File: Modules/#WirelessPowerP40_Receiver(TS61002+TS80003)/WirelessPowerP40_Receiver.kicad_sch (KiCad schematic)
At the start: 123 parts, among them J2 I2C, J3 I2C, J4 Coil Therm, J5 COIL 20uH, J6 Conn_01x02_Male, J7 Conn_01x02_Male, U1 TS30041, U2 TS94033, U3 74LVC1G66, U4 TS61002, U5 TS80003, U6 BSC0993ND, U7 BSC0993ND, U8 max31740, U9 CSD16406Q3

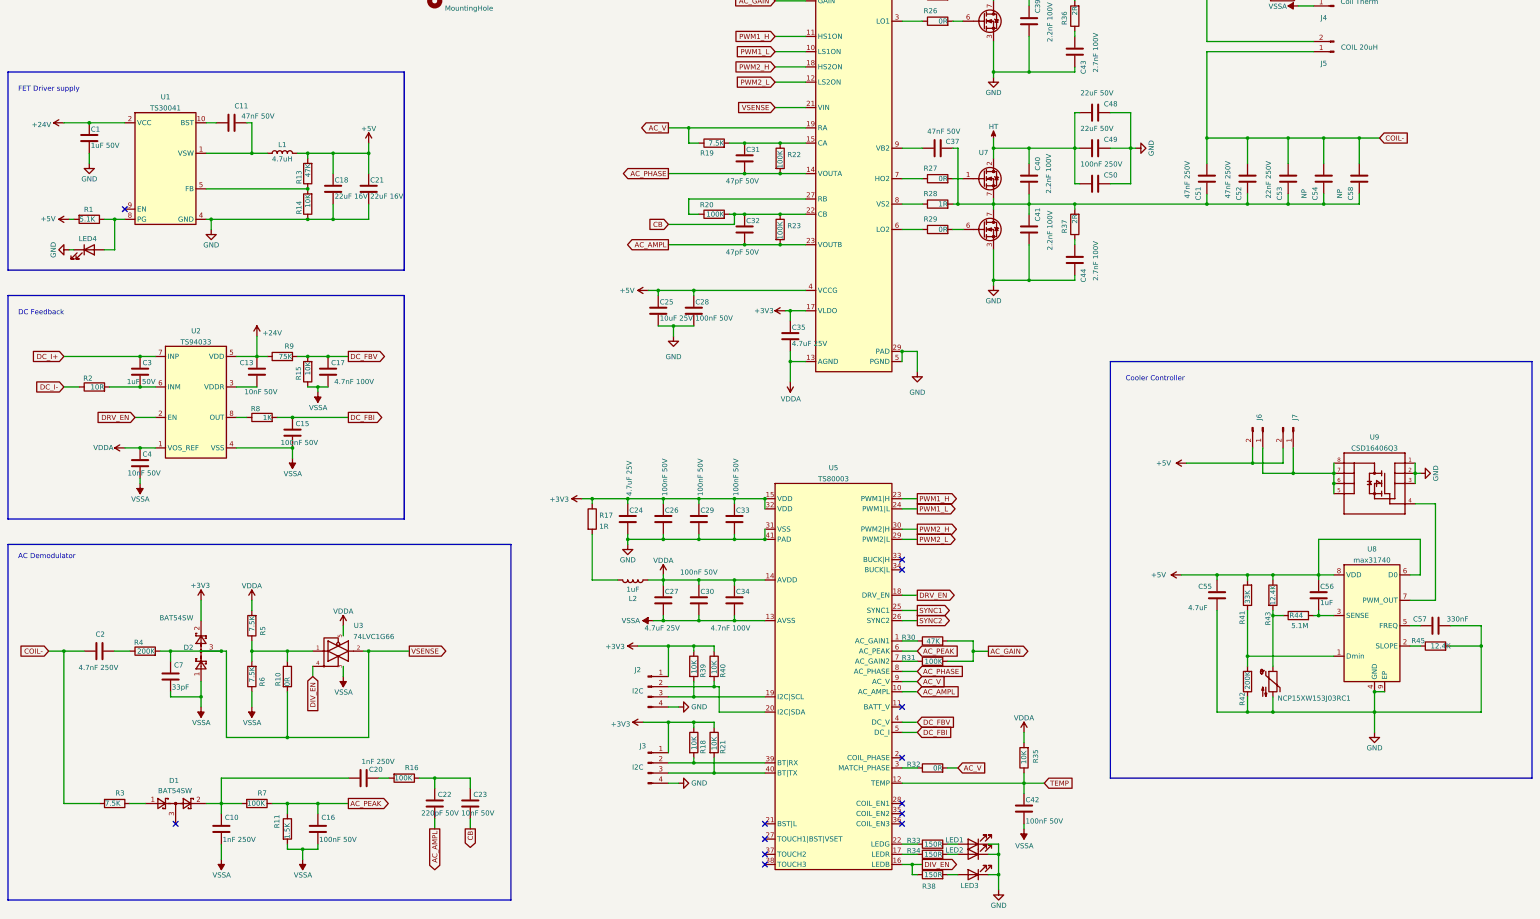
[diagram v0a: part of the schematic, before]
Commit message: WirelessPowerP40_Transmitter optimization
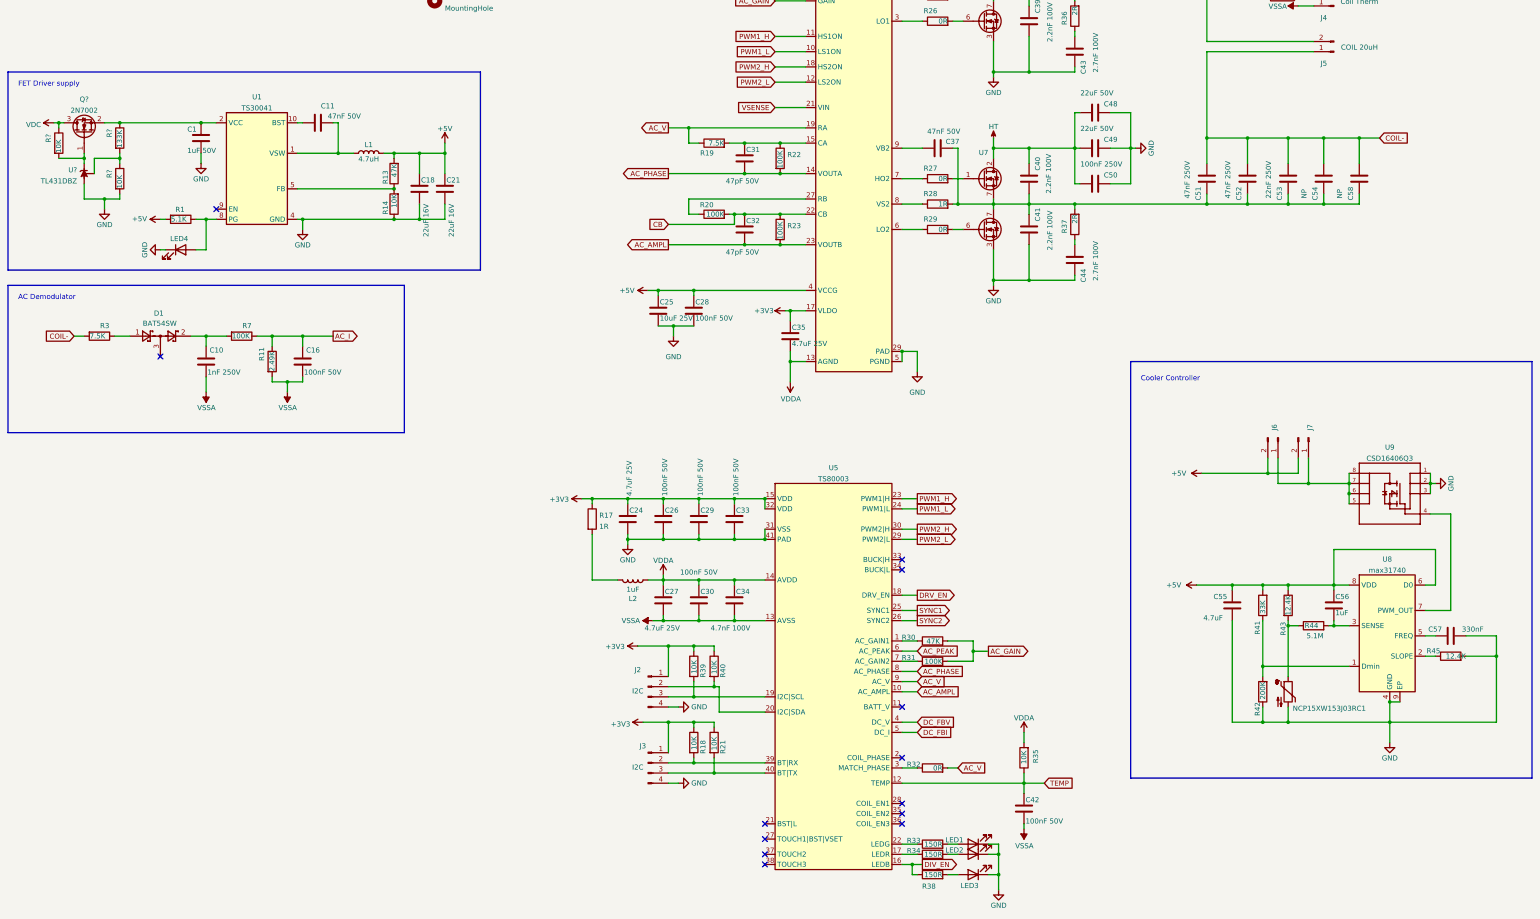
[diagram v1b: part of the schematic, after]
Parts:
- removed C13, C23, C4: 10nF 50V, Capacitor_SMD:C_0402_1005Metric, symbol Device:C
- removed C15: 100nF 50V, Capacitor_SMD:C_0402_1005Metric, symbol Device:C
- removed C17: 4.7nF 100V, Capacitor_SMD:C_0402_1005Metric, symbol Device:C
- removed C2: 4.7nF 250V, Capacitor_SMD:C_0603_1608Metric, symbol Device:C
- removed C20: 1nF 250V, Capacitor_SMD:C_0603_1608Metric, symbol Device:C
- removed C22: 220pF 50V, Capacitor_SMD:C_0402_1005Metric, symbol Device:C
- removed C3: 1uF 50V, Capacitor_SMD:C_0402_1005Metric, symbol Device:C
- removed C7: 33pF, Capacitor_SMD:C_0402_1005Metric, symbol Device:C
- removed D2: BAT54SW, Package_TO_SOT_SMD:SOT-323_SC-70, symbol Diode:BAT54SW
- removed R10: 0R, Resistor_SMD:R_0402_1005Metric, symbol Device:R
- removed R15: 10K, Resistor_SMD:R_0402_1005Metric, symbol Device:R
- removed R16: 100K, Resistor_SMD:R_0603_1608Metric, symbol Device:R
- removed R2: 10R, Resistor_SMD:R_0402_1005Metric, symbol Device:R
- removed R4: 200K, Resistor_SMD:R_0402_1005Metric, symbol Device:R
- removed R5, R6: 7.5K, Resistor_SMD:R_0402_1005Metric, symbol Device:R
- removed R8: 1K, Resistor_SMD:R_0402_1005Metric, symbol Device:R
- removed R9: 75K, Resistor_SMD:R_0402_1005Metric, symbol Device:R
- removed U2: TS94033, Package_TO_SOT_SMD:SOT-23-8, symbol TS:TS94033
- removed U3: 74LVC1G66, Package_SO:TSOP-5_1.65x3.05mm_P0.95mm, symbol 74xGxx:74LVC1G66
- added Q?: 2N7002, Package_TO_SOT_SMD:SOT-23, symbol Transistor_FET:2N7002
- added R? (x2): 10K, Resistor_SMD:R_0402_1005Metric, symbol Device:R
- added R?: 133K, Resistor_SMD:R_0402_1005Metric, symbol Device:R
- added U?: TL431DBZ, Package_TO_SOT_SMD:SOT-23, symbol Reference_Voltage:TL431DBZ
- R11: value 1.5K -> 2.49K
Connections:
- net AC_PEAK: no longer C16.1, R11.1, R7.1
- net GND: now also R?.2, U?.3 (A)
- net +24V renamed VCC
- net VCC: now also Q?.2 (S), R?.1
- new net: R?.1, R?.2, U?.2 (REF)
- new net: Q?.1 (G), R?.2, U?.1 (K)
- new net AC_I: C16.1, R11.1, R7.1
- new net VDC: Q?.3 (D), R?.1
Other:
- note removed: "DC Feedback"
- moved on the sheet: C1, C10, C11, C16, C18, C21, C55, C56, C57, D1, J6, J7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

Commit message: continue..
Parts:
- removed J4: Coil Therm, Connector_PinHeader_2.00mm:PinHeader_1x02_P2.00mm_Vertical, symbol Connector:Conn_01x02_Male
- removed LED3: LED, LED_SMD:LED_0402_1005Metric, symbol Device:LED
- added C12, C9: 15nF 50V, Capacitor_SMD:C_0402_1005Metric, symbol Device:C
- added C13, C14, C17, C19, C7: 100nF 50V, Capacitor_SMD:C_0402_1005Metric, symbol Device:C
- added C15, C20: 1uF 50V, Capacitor_SMD:C_0402_1005Metric, symbol Device:C
- added C2, C3: 22uF 50V, Capacitor_SMD:C_0805_2012Metric, symbol Device:C
- added C22: 10nF 50V, Capacitor_SMD:C_0402_1005Metric, symbol Device:C
- added C23: 100nF, Capacitor_SMD:C_0402_1005Metric, symbol Device:C
- added C4, C6: 1nF 250V, Capacitor_SMD:C_0603_1608Metric, symbol Device:C
- added C5: 10pF 50V, Capacitor_SMD:C_0402_1005Metric, symbol Device:C
- added C59, C60, C62, C63: 10uF, Capacitor_SMD:C_1206_3216Metric, symbol Device:C
- added C61: 330pF, Capacitor_SMD:C_0402_1005Metric, symbol Device:C
- added C8: 4.7uF 25V, Capacitor_SMD:C_0402_1005Metric, symbol Device:C
- added D2: BAT54SW, Package_TO_SOT_SMD:SOT-323_SC-70, symbol Diode:BAT54SW
- added D3: BAS21-03W, Package_TO_SOT_SMD:SOT-23, symbol Diode:BAS21
- added J1: Conn_01x02_Male, Connector_PinHeader_2.00mm:PinHeader_1x02_P2.00mm_Vertical, symbol Connector:Conn_01x02_Male
- added L3: EE55100, symbol Device:L_Ferrite_Coupled_1423
- added L4: 22uH, Inductor_SMD:L_Wuerth_HCI-1030, symbol Device:L
- added Q2, Q3, Q4: 2N7002, Package_TO_SOT_SMD:SOT-23, symbol Transistor_FET:2N7002
- added Q5: BSC100N06L, Package_TO_SOT_SMD:TDSON-8-1, symbol Transistor_FET:BSC100N10NSFG
- added Q6: BSC028N06L, Package_TO_SOT_SMD:TDSON-8-1, symbol Transistor_FET:BSC026N08NS5
- added R10, R12, R60, R61, R8, R9: 20K, Resistor_SMD:R_0402_1005Metric, symbol Device:R
- added R15: 20R, Resistor_SMD:R_0603_1608Metric, symbol Device:R
- added R16: 200K, Resistor_SMD:R_0402_1005Metric, symbol Device:R
- added R46: 75K, Resistor_SMD:R_0402_1005Metric, symbol Device:R
- added R47, R48, R55, R57, R62: 10K, Resistor_SMD:R_0402_1005Metric, symbol Device:R
- added R49, R50, R51, R52, R6: 0R, Resistor_SMD:R_0402_1005Metric, symbol Device:R
- added R53: 715K, Resistor_SMD:R_0402_1005Metric, symbol Device:R
- added R54: 133K, Resistor_SMD:R_0402_1005Metric, symbol Device:R
- added R56, R58: 1R, Resistor_SMD:R_0402_1005Metric, symbol Device:R
- added R59: 3R3, Resistor_SMD:R_0402_1005Metric, symbol Device:R
- added R63: 4.99K, Resistor_SMD:R_0402_1005Metric, symbol Device:R
- added R64: 9.09K, Resistor_SMD:R_0402_1005Metric, symbol Device:R
- added R65, R67: 1K, Resistor_SMD:R_0402_1005Metric, symbol Device:R
- added R66: 34K, Resistor_SMD:R_0402_1005Metric, symbol Device:R
- added R68: 499K, Resistor_SMD:R_0402_1005Metric, symbol Device:R
- added U3: SC506, Package_DFN_QFN:QFN-20-1EP_3x3mm_P0.4mm_EP1.65x1.65mm, symbol TS:SC506
- C32: value 47pF 50V -> 1nF
- C53: value 22nF 250V -> 10nF 250V
- C58: value NP -> 22nF; footprint Capacitor_SMD:C_1210_3225Metric -> Capacitor_SMD:C_0402_1005Metric
- D1: value BAT54SW -> BAS101S,215; footprint Package_TO_SOT_SMD:SOT-323_SC-70 -> Package_TO_SOT_SMD:SOT-23
- J5: value COIL 20uH -> COIL 24uH
- R11: value 2.49K -> 1.5K
- R19: value 7.5K -> 10K
- R20, R23: value 100K -> 7.5K
- R22: value 100K -> 10K
- R24, R26, R27, R29: value 0R -> 1R
- R25, R28: value 1R -> 0R
- R30: value 47K -> 100K
- R31: value 100K -> 200R
- R32: value 0R -> 10K
- R38: value 150R -> 4.7K
- gave numbers to parts that had none: 5
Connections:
- net VSSA is gone; now on net GND: C10.2, C16.2, C27.2, C30.2, C34.2, C42.2, R11.2, U5.13 (AVSS)
- net +3V3: now also D2.2
- net +5V: now also C15.2, C17.2, U3.13 (VDDP), U3.14 (PSV), U3.3 (VDDA)
- net AC_I: now also U5.6 (AC_I); no longer C16.1, R11.1, R7.1
- net AC_PEAK: now also C16.1, R11.1, R7.1; no longer U5.6 (AC_PEAK)
- net COIL-: no longer C58.1
- net GND: now also R23.1, R30.2, C13.1, C14.2, C15.1, C17.1, C19.1, C2.1, C20.1, C22.1, C3.1, C5.1, C59.1, C60.1, C62.1, C63.1, C7.2, C8.2, D2.1, J1.1 (Pin_1), Q2.2 (S), Q3.2 (S), Q4.2 (S), Q6.1 (S), Q6.2 (S), Q6.3 (S), R12.1, R47.1, R53.1, R55.1, R61.2, R65.2, R67.2, R9.1, U3.11 (PGND), U3.18 (AGND), U3.20 (ENL), U3.21 (EP); no longer C25.2, C28.2
- net HT: now also Q1.3 (D), R2.1, R31.1, C2.2, C3.2, Q5.5 (D), R54.2, R68.2, U3.5 (VIN)
- net PWM1_H: now also R49.2
- net PWM1_L: now also R52.2
- net PWM2_H: now also R51.2
- net PWM2_L: now also R50.2
- net TEMP: now also U5.11 (TEMP), J1.2 (Pin_2); no longer U5.12 (TEMP)
- net VDC: now also C58.2, C59.2, C60.2, C61.2, C62.2, C63.2, L4.2, R46.2, R64.1, R66.1; no longer Q1.3 (D), R2.1
- net VDDA: now also C25.2, C28.2, R20.2, R16.2, R48.2
- net at C37.2, C40.1, C41.2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: now also L3.1, R10.1; no longer C51.2, C52.2, C53.2, C54.2, C58.2
- net VAC1: now reaches C36.2, C38.1, C39.2, J5.2 (Pin_2), R25.2, R36.2, U6.7
- net VAC1: now also C4.1, C6.1, C9.1, R8.1
- net at R24.2, U6.1: now also R8.2
- net at R26.2, U6.6: now also R9.2
- net AC_I_1: now reaches U5.7 (AC_I_1)
- net AC_I_1: now also R19.1, U4.19 (RA); no longer R31.1
- net at R29.2, U7.6: now also R12.2
- net EN_MOD: now reaches R30.1
- net EN_MOD: now also U5.25 (EN_MOD), Q2.1 (G), Q4.1 (G); no longer U5.1 (AC_GAIN1)
- net at U5.22 (ACMP1_OUT): now also R49.1, R50.1; no longer R33.1
- net at U5.28 (ACMP2_OUT): now also R51.1, R52.1
- net at R32.1: now also U5.35 (AC_GAIN1); no longer U5.3 (MATCH_PHASE)
- net at U5.36 (AC_GAIN2): now also R38.1
- net MIN_LD: now reaches U5.37 (EN_MINLD)
- net MIN_LD: now also Q3.1 (G)
- net at U4.27 (RB): no longer R20.1
- net EN_GAIN: now reaches R38.2
- net EN_GAIN: now also R32.2, U4.24 (GAIN)
- net at R27.2, U7.1: now also R10.2
- removed net AC_AMPL: C32.2, R23.2, U4.23 (VOUTB), U5.10 (AC_AMPL)
- removed net AC_GAIN: R30.2, R31.2, U4.24 (GAIN)
- net AC_PHASE renamed AC_I_2
- net AC_I_2: now also U5.3 (AC_I_2); no longer U5.8 (AC_PHASE)
- removed net AC_V: R19.1, R32.2, U4.19 (RA), U5.9 (AC_V)
- removed net CB: C32.1, R20.2, R23.1, U4.22 (CB)
- net DC_FBI: no longer names the net of U5.5 (DC_I)
- net DC_FBV renamed DC_V
- net DC_V: now also C13.2, R46.1, R47.2
- net DIV_EN: no longer names the net of U5.16 (LEDG)
- net DIV_EN: now also R33.1; no longer R38.1
- net DRV_EN renamed EN_DRV
- net SYNC1: no longer names the net of U4.20 (SYNC1)
- net SYNC1: no longer U5.25 (SYNC1)
- net SYNC2: no longer names the net of U4.25 (SYNC2)
- net SYNC2: no longer U5.26 (SYNC2)
- net VSENSE renamed ISENSE
- net ISENSE: now also C5.2, D2.3, L3.3, R15.2
- new net: D3.3 (K), L4.1, Q5.1 (S), Q5.2 (S), Q5.3 (S), Q6.5 (D), R57.1, R59.1, R60.2, R62.2, U3.10 (LX)
- new net: Q5.4 (G), R56.1, R60.1
- new net: C32.2, C58.1, R62.1, R63.1
- new net: Q3.3 (D), R31.2
- new net: C32.1, C61.1, R66.2, R67.1, R68.1, U3.1 (FB)
- new net: Q6.4 (G), R58.1, R61.1
- new net: R58.2, U3.12 (DL)
- new net: R6.1, U4.22 (CB), U4.23 (VOUTB)
- new net: R64.2, R65.1, U3.2 (VOUT)
- new net: R57.2, U3.16 (LIMI)
- new net: R53.2, U3.19 (TON)
- new net: C20.2, U3.4 (VLDO)
- new net: C22.2, U3.6 (SS)
- new net: C23.1, U3.8 (BST)
- new net: R56.2, U3.9 (DH)
- new net: C23.2, R59.2
- new net: C9.2, Q2.3 (D)
- new net: D3.1 (A), R63.2
- new net: C12.2, Q4.3 (D)
- new net ACMPREF: C14.1, R48.1
- new net EN_LOAD: U3.17 (EN), U5.26 (EN_LOAD)
- new net PDC_V: C19.2, R54.1, R55.2, U5.1 (PDC_V)
- new net VAC2: C12.1, C4.2, C51.2, C52.2, C53.2, C54.2, C6.2, L3.4
- new net VACC_MID: C7.1, C8.1, L3.2, R15.1, R16.1, R20.1, R23.2, R6.2
- no-connect marks 13 -> 15
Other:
- moved on the sheet: C1, C10, C11, C16, C18, C21, C24, C25, C26, C27, C28, C29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
